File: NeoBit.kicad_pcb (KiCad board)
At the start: 2 copper layers, 77.5 x 45.7 mm, 22 parts, among them J1 AudioJack3_Ground, J2 Barrel_Jack_MountingPin, J3 Qwiic, J4 DotStars, J5 microbit_edge_connector, J6 NeoPixels, U1 74AHCT125, U2 MCP1702-3302E_TO92, U3 MCP1702-5002E_TO92

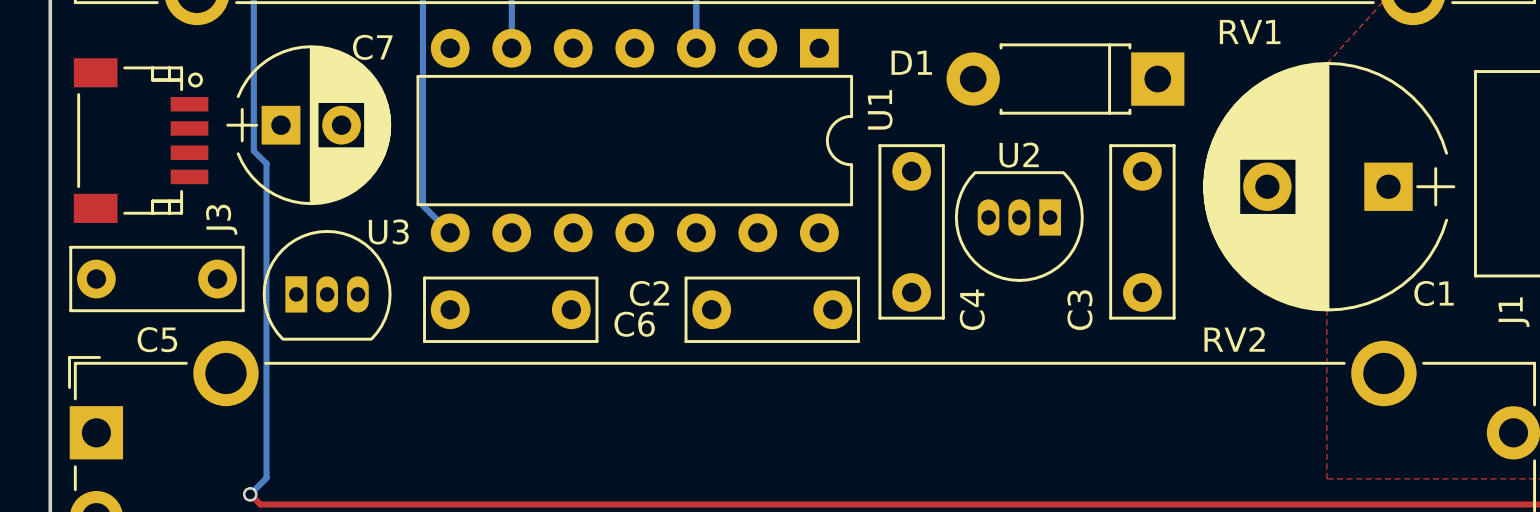
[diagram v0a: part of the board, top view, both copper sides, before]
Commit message: Added some more tracks.
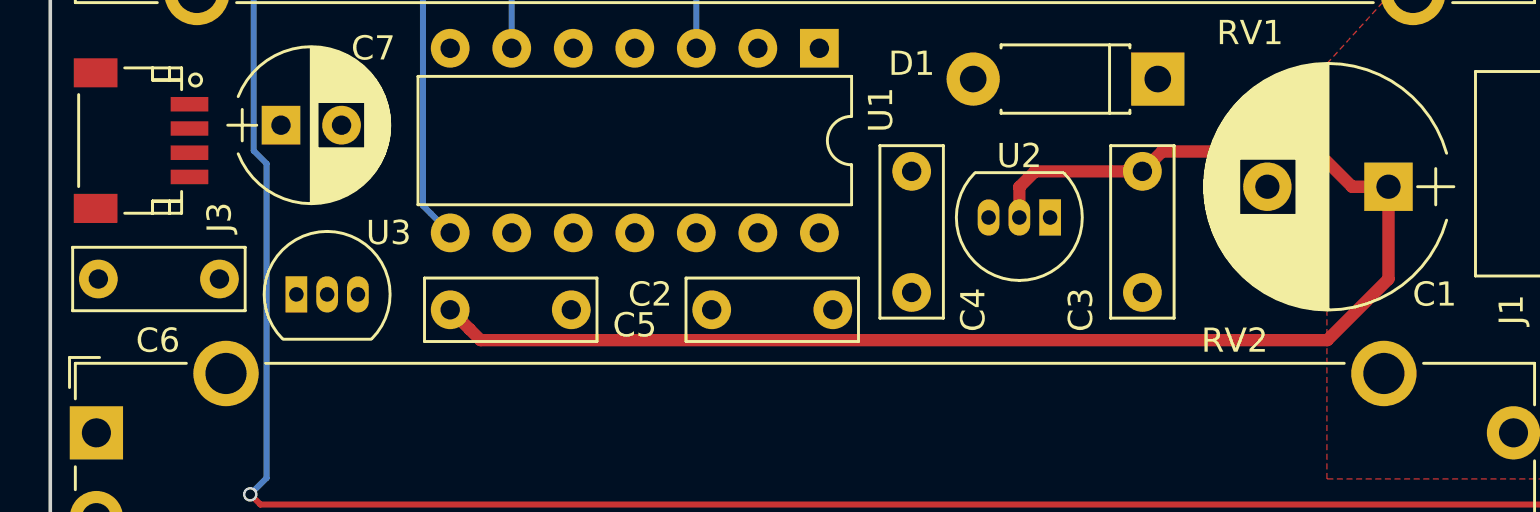
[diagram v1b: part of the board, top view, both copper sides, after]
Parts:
- moved C5 14.7 mm to (135.3, 116.8)
- moved C6 9.61 mm to (125.7, 115.6), turned to 180 degrees
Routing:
- net +VDC: track 0.00 -> 61.8 mm
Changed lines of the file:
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@@
   (general
     (links 81)
-    (no_connects 57)
+    (no_connects 46)
     (area 118.669999 83.744999 186.130001 129.615001)
     (thickness 1.6)
     (drawings 14)
-    (tracks 54)
+    (tracks 67)
     (zones 0)
     (modules 22)
@@
   )
   (setup
-    (last_trace_width 0.25)
+    (last_trace_width 0.508)
     (user_trace_width 0.508)
     (user_trace_width 1.016)
@@
   )
   (module Capacitors_THT:C_Rect_L7.0mm_W2.5mm_P5.00mm (layer F.Cu)
-    (at 120.65 115.57)
+    (at 135.255 116.84)
     (descr "C, Rect series, Radial, pin pitch=5.00mm, , length*width=7*2.5mm^2, Capacitor")
     (tags "C Rect series Radial pin pitch 5.00mm  length 7mm width 2.5mm Capacitor")
-    (fp_text reference C5 (at 2.54 2.54) (layer F.SilkS)
+    (fp_text reference C5 (at 7.62 0.635) (layer F.SilkS)
       (effects (font (size 1 1) (thickness 0.15)))
     )
@@
   )
   (module Capacitors_THT:C_Rect_L7.0mm_W2.5mm_P5.00mm (layer F.Cu)
-    (at 135.255 116.84)
+    (at 125.73 115.57 180)
     (descr "C, Rect series, Radial, pin pitch=5.00mm, , length*width=7*2.5mm^2, Capacitor")
     (tags "C Rect series Radial pin pitch 5.00mm  length 7mm width 2.5mm Capacitor")
-    (fp_text reference C6 (at 7.62 0.635) (layer F.SilkS)
-      (effects (font (size 1 1) (thickness 0.15)))
-    )
-    (fp_text value 1µF (at 2.5 2.56) (layer F.Fab)
+    (fp_text reference C6 (at 2.54 -2.54 180) (layer F.SilkS)
+      (effects (font (size 1 1) (thickness 0.15)))
+    )
+    (fp_text value 1µF (at 2.5 2.56 180) (layer F.Fab)
       (effects (font (size 1 1) (thickness 0.15)))
     )
@@
     (fp_line (start 6.35 1.6) (end 6.35 -1.6) (layer F.CrtYd) (width 0.05))
     (fp_line (start 6.35 -1.6) (end -1.35 -1.6) (layer F.CrtYd) (width 0.05))
-    (fp_text user %R (at 2.5 0) (layer F.Fab)
-      (effects (font (size 1 1) (thickness 0.15)))
-    )
-    (pad 1 thru_hole circle (at 0 0) (size 1.6 1.6) (drill 0.8) (layers *.Cu *.Mask)
+    (fp_text user %R (at 2.5 0 180) (layer F.Fab)
+      (effects (font (size 1 1) (thickness 0.15)))
+    )
+    (pad 1 thru_hole circle (at 0 0 180) (size 1.6 1.6) (drill 0.8) (layers *.Cu *.Mask)
       (net 1 +5V))
-    (pad 2 thru_hole circle (at 5 0) (size 1.6 1.6) (drill 0.8) (layers *.Cu *.Mask)
+    (pad 2 thru_hole circle (at 5 0 180) (size 1.6 1.6) (drill 0.8) (layers *.Cu *.Mask)
       (net 2 GND))
     (model ${KISYS3DMOD}/Capacitors_THT.3dshapes/C_Rect_L7.0mm_W2.5mm_P5.00mm.wrl
@@
   (segment (start 174.464002 97.155) (end 145.415 97.155) (width 0.25) (layer F.Cu) (net 8))
   (via (at 145.415 97.155) (size 0.6) (drill 0.4) (layers F.Cu B.Cu) (net 8))
+  (segment (start 173.99 115.57) (end 171.465999 118.094001) (width 0.508) (layer F.Cu) (net 9))
+  (segment (start 171.465999 118.094001) (end 136.509001 118.094001) (width 0.508) (layer F.Cu) (net 9))
+  (segment (start 136.509001 118.094001) (end 136.054999 117.639999) (width 0.508) (layer F.Cu) (net 9))
+  (segment (start 136.054999 117.639999) (end 135.255 116.84) (width 0.508) (layer F.Cu) (net 9))
+  (segment (start 173.99 111.76) (end 173.99 115.57) (width 0.508) (layer F.Cu) (net 9))
+  (segment (start 163.83 111.125) (end 159.397 111.125) (width 0.508) (layer F.Cu) (net 9))
+  (segment (start 159.397 111.125) (end 158.75 111.772) (width 0.508) (layer F.Cu) (net 9))
+  (segment (start 158.75 111.772) (end 158.75 113.03) (width 0.508) (layer F.Cu) (net 9))
+  (segment (start 173.99 111.76) (end 172.482 111.76) (width 0.508) (layer F.Cu) (net 9))
+  (segment (start 172.482 111.76) (end 171.027999 110.305999) (width 0.508) (layer F.Cu) (net 9))
+  (segment (start 171.027999 110.305999) (end 164.649001 110.305999) (width 0.508) (layer F.Cu) (net 9))
+  (segment (start 164.649001 110.305999) (end 164.629999 110.325001) (width 0.508) (layer F.Cu) (net 9))
+  (segment (start 164.629999 110.325001) (end 163.83 111.125) (width 0.508) (layer F.Cu) (net 9))
   (segment (start 186.055 103.505) (end 183.515 103.505) (width 0.25) (layer F.Cu) (net 15))
   (segment (start 186.055 100.33) (end 186.055 103.505) (width 0.25) (layer B.Cu) (net 15))
